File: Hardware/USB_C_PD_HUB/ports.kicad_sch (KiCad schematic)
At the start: 1 part, among them J1 USB_C_Receptacle

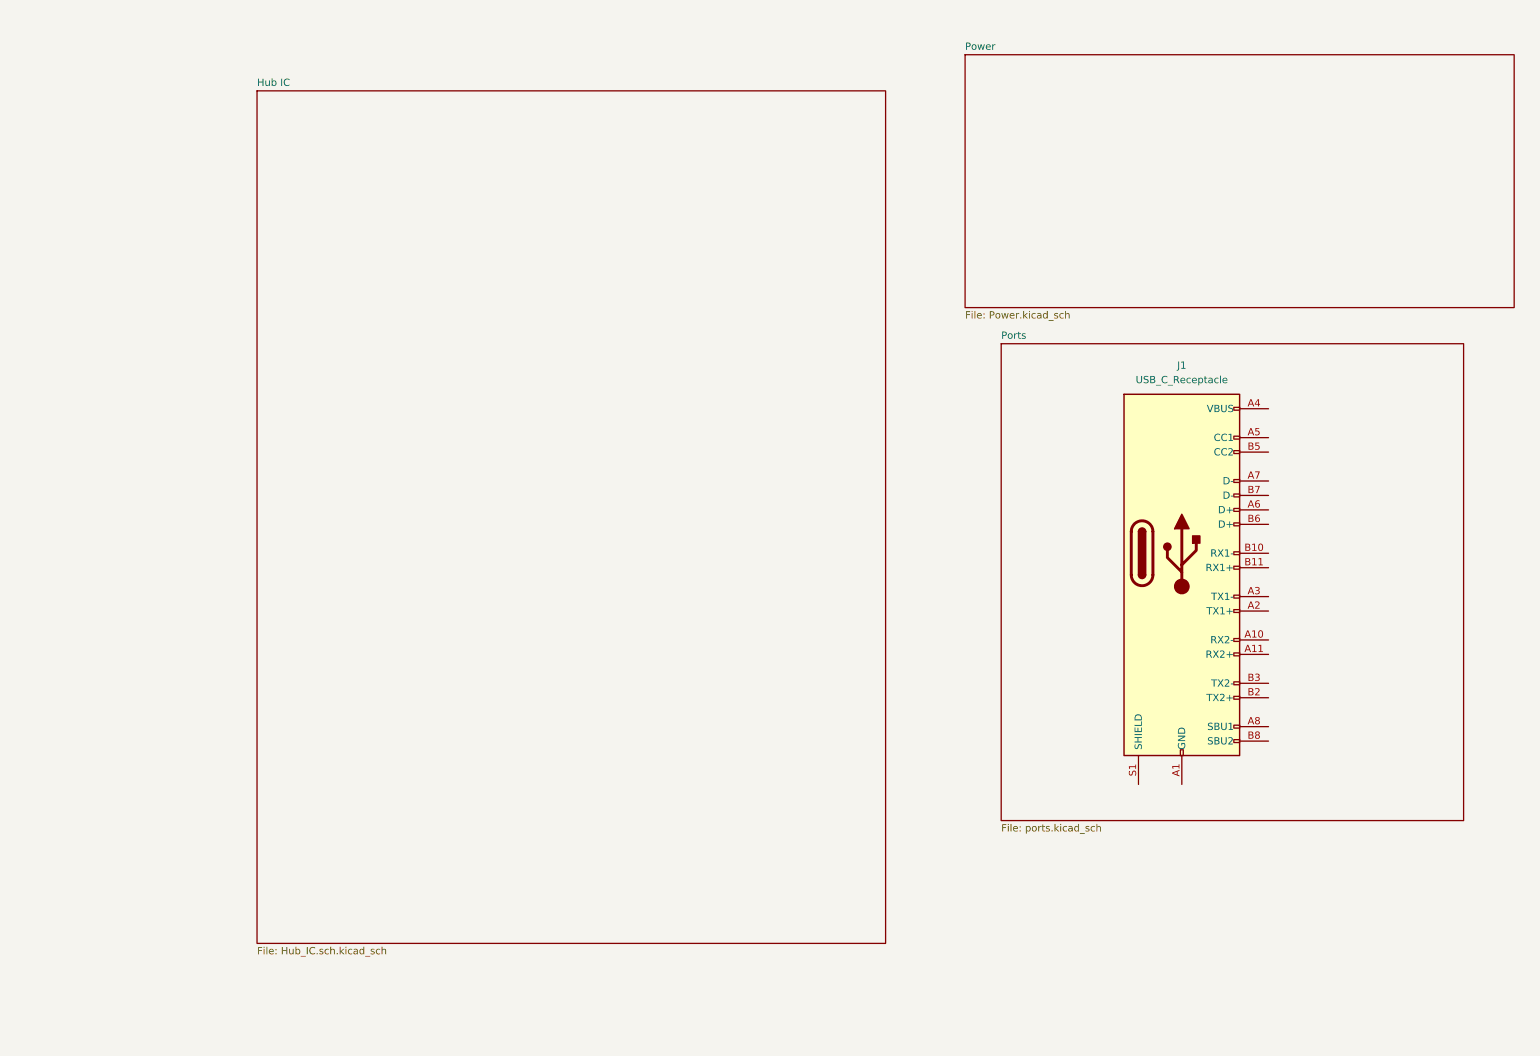
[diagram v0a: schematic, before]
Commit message: Sch stuff
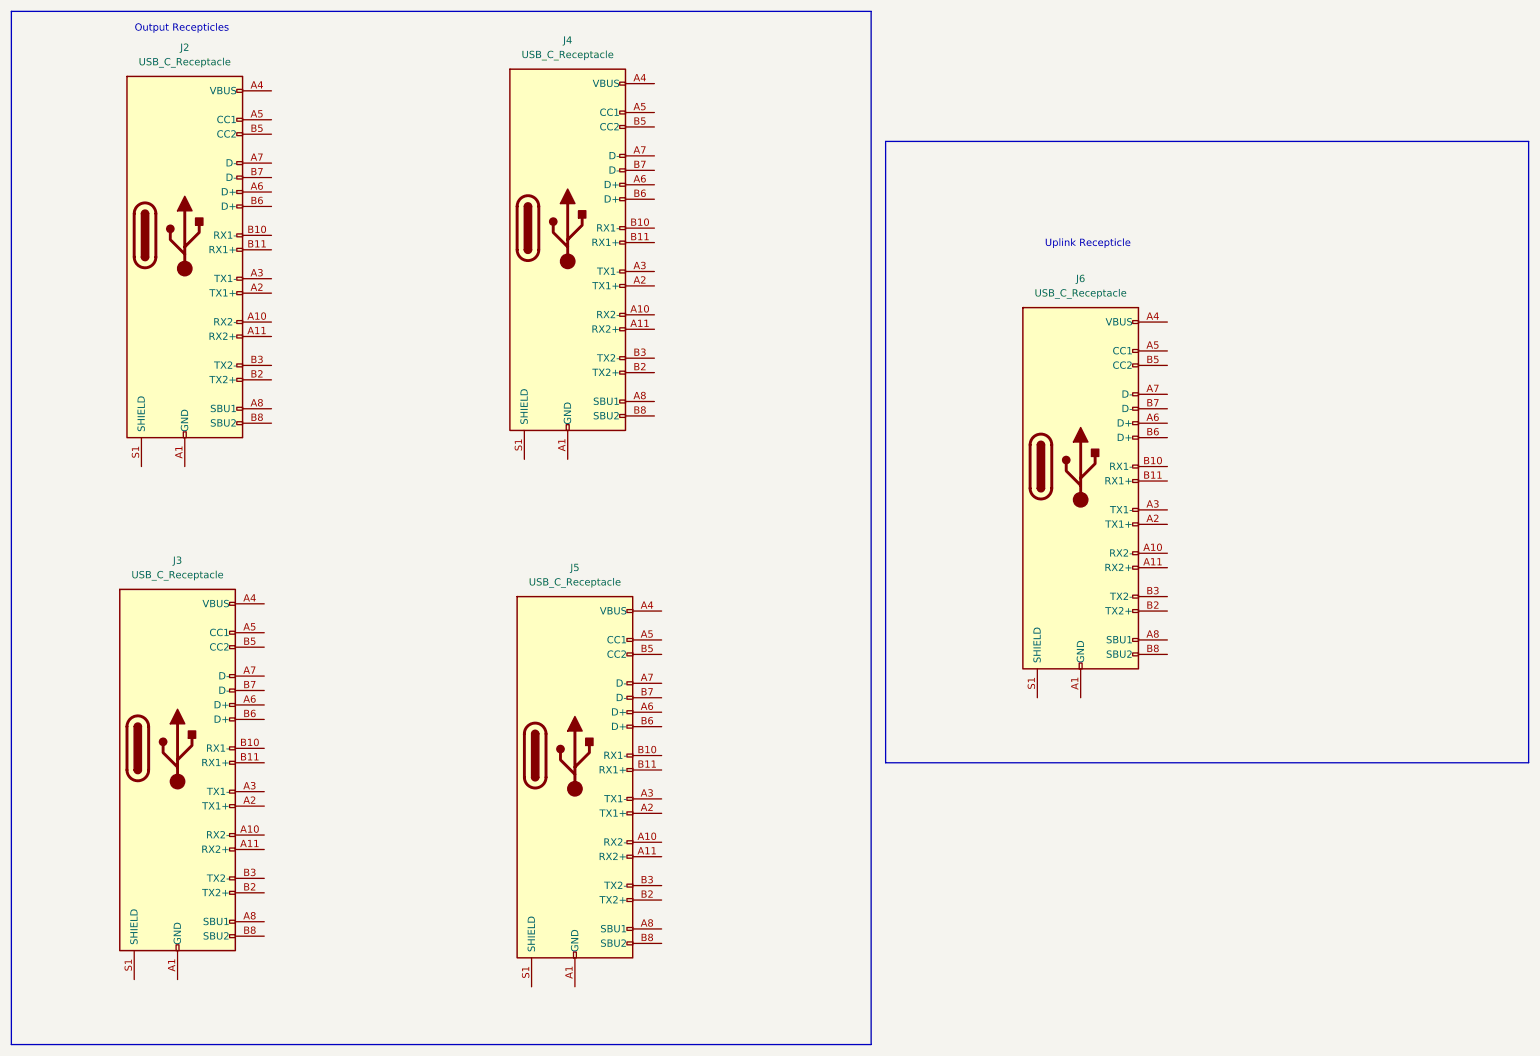
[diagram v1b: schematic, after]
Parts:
- removed J1: USB_C_Receptacle, Connector_USB:USB_C_Receptacle_GCT_USB4115-03-C, symbol Connector:USB_C_Receptacle
- added J2, J3, J4, J5, J6: USB_C_Receptacle, Connector_USB:USB_C_Receptacle_GCT_USB4115-03-C, symbol Connector:USB_C_Receptacle
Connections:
- new net: J4.A1 (GND), J4.A12 (GND), J4.B1 (GND), J4.B12 (GND)
- new net: J4.A4 (VBUS), J4.A9 (VBUS), J4.B4 (VBUS), J4.B9 (VBUS)
- new net: J6.A1 (GND), J6.A12 (GND), J6.B1 (GND), J6.B12 (GND)
- new net: J6.A4 (VBUS), J6.A9 (VBUS), J6.B4 (VBUS), J6.B9 (VBUS)
- new net: J5.A1 (GND), J5.A12 (GND), J5.B1 (GND), J5.B12 (GND)
- new net: J5.A4 (VBUS), J5.A9 (VBUS), J5.B4 (VBUS), J5.B9 (VBUS)
- new net: J3.A1 (GND), J3.A12 (GND), J3.B1 (GND), J3.B12 (GND)
- new net: J3.A4 (VBUS), J3.A9 (VBUS), J3.B4 (VBUS), J3.B9 (VBUS)
- new net: J2.A1 (GND), J2.A12 (GND), J2.B1 (GND), J2.B12 (GND)
- new net: J2.A4 (VBUS), J2.A9 (VBUS), J2.B4 (VBUS), J2.B9 (VBUS)
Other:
- removed sheet Hub IC
- removed sheet Ports
- removed sheet Power
- note added: "Output Recepticles"
- note added: "Uplink Recepticle"
